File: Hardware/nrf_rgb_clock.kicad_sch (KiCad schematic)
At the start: 23 parts, among them U1 NRF54L15-CAAA-Rx, Y1 32MHz

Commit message: progressed layout
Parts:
- added C10, C11: 4u7 100VDC, Capacitor_SMD:C_1206_3216Metric, symbol Device:C_Small
- added C12: 100n 100VDC, Capacitor_SMD:C_0805_2012Metric, symbol Device:C_Small
- added C13, C14: 22u 6.3V, Capacitor_SMD:C_0805_2012Metric, symbol Device:C_Small
- added C15: 15p, Capacitor_SMD:C_0805_2012Metric, symbol Device:C_Small
- added C16: 22n, Capacitor_SMD:C_0805_2012Metric, symbol Device:C_Small
- added C17, C18: ?p, Capacitor_SMD:C_0201_0603Metric, symbol Device:C_Small
- added D174: ACDBMS2100-HF, Diode_SMD:D_SOD-123F, symbol Device:D_Schottky_Small_Filled
- added J1: Conn_01x02, ProjectFootprints:SHDR4W113P700X508_2X2_1039X1200X1200P, symbol Connector_Generic:Conn_01x02
- added L5: 10u, ProjectFootprints:NRS5040T3R3NMGJV, symbol Device:L_Small
- added R1: 0R, Resistor_SMD:R_0805_2012Metric, symbol Device:R_Small
- added R2: 210k, Resistor_SMD:R_0805_2012Metric, symbol Device:R_Small
- added R3: 68k, Resistor_SMD:R_0805_2012Metric, symbol Device:R_Small
- added R4: 47k, Resistor_SMD:R_0805_2012Metric, symbol Device:R_Small
- added TP1, TP2: TestPoint, TestPoint:TestPoint_THTPad_2.0x2.0mm_Drill1.0mm, symbol Connector:TestPoint
- added U2: MP4562, ProjectFootprints:MP4562, symbol ProjectSymbols:MP4562
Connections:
- net GND: now also C10.2, C11.2, C13.2, C14.2, C16.2, C17.2, C18.2, D174.2 (A), J1.2 (Pin_2), R3.2, R4.2, TP2.1, U2.2 (GND)
- net NRF_RF: now also AE1.1 (FEED), L2.2
- net NRF_XC1: now also Y1.1, C17.1; no longer Y1.3
- net NRF_XC2: now also Y1.3, C18.1; no longer Y1.1
- new net: C12.2, D174.1 (K), L5.1, U2.7 (SW)
- new net: C15.2, R2.2, R3.1, U2.4 (FB)
- new net: R4.1, U2.3 (FREQ)
- new net: C12.1, U2.8 (BST)
- new net: C16.1, U2.1 (SS)
- new net: R1.1, U2.5 (EN)
- new net +3V3: C13.1, C14.1, C15.1, L5.2, R2.1, TP1.1
- new net V_EXT: C10.1, C11.1, J1.1 (Pin_1), R1.2, U2.6 (VIN)
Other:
- note added: "3V3 BUCK"
- note added: "ACDC Converter 48-24Vin"
- note removed: "Power"
- moved on the sheet: AE1, C1, C2, C3, C4, C5, C6, C7, C8, C9, D116, D117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

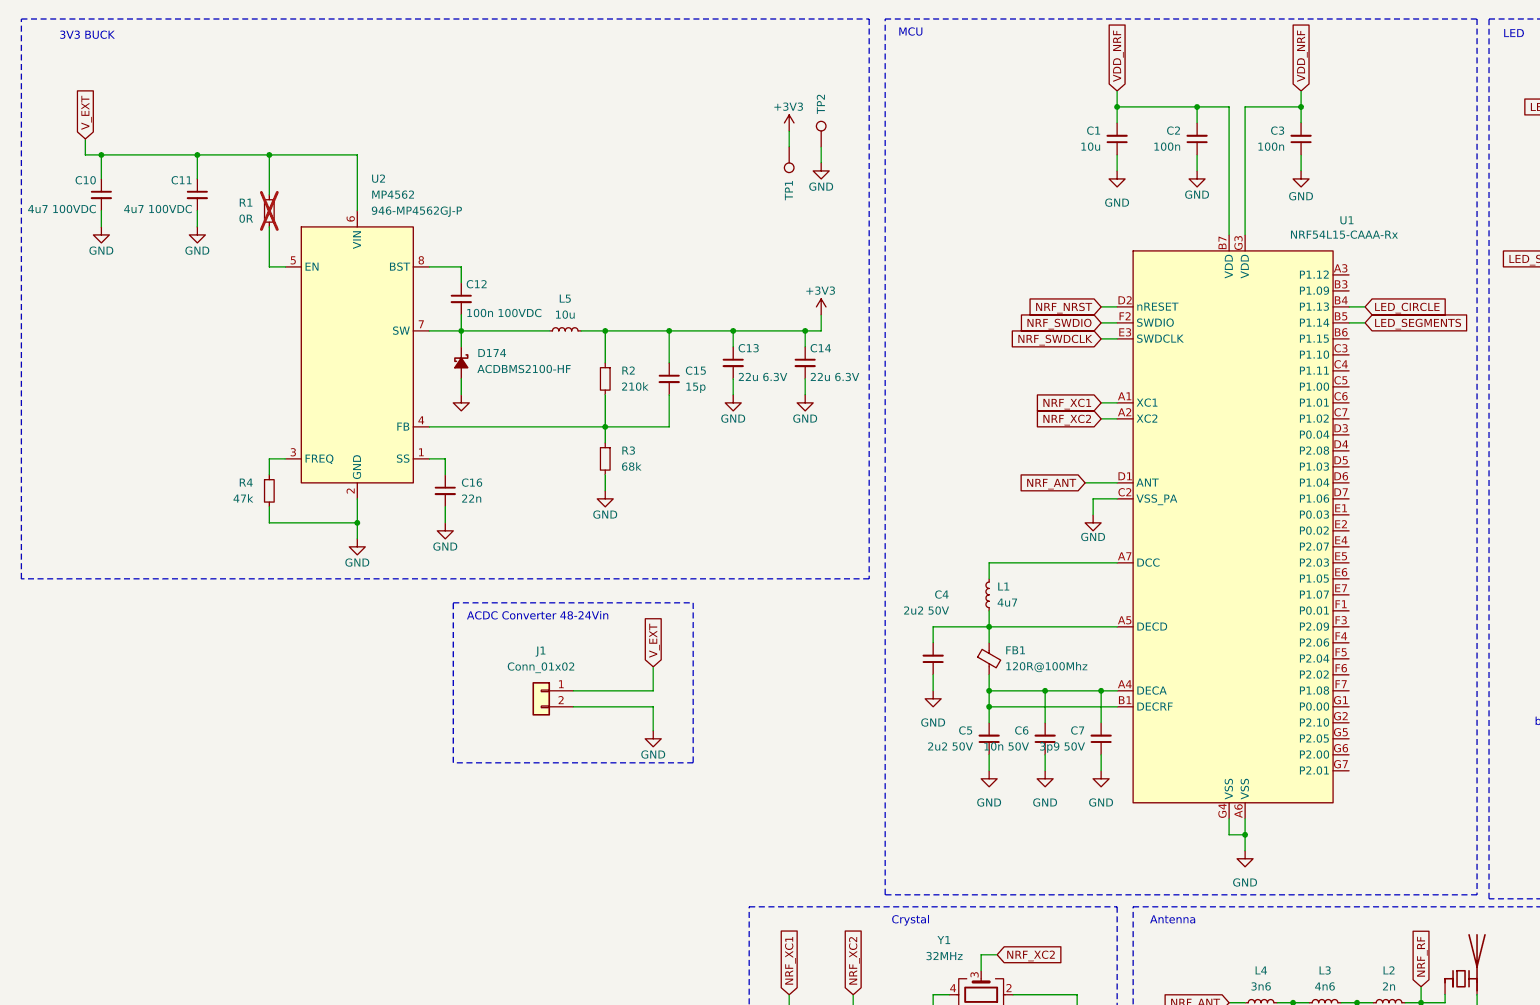
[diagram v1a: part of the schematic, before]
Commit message: layout progress
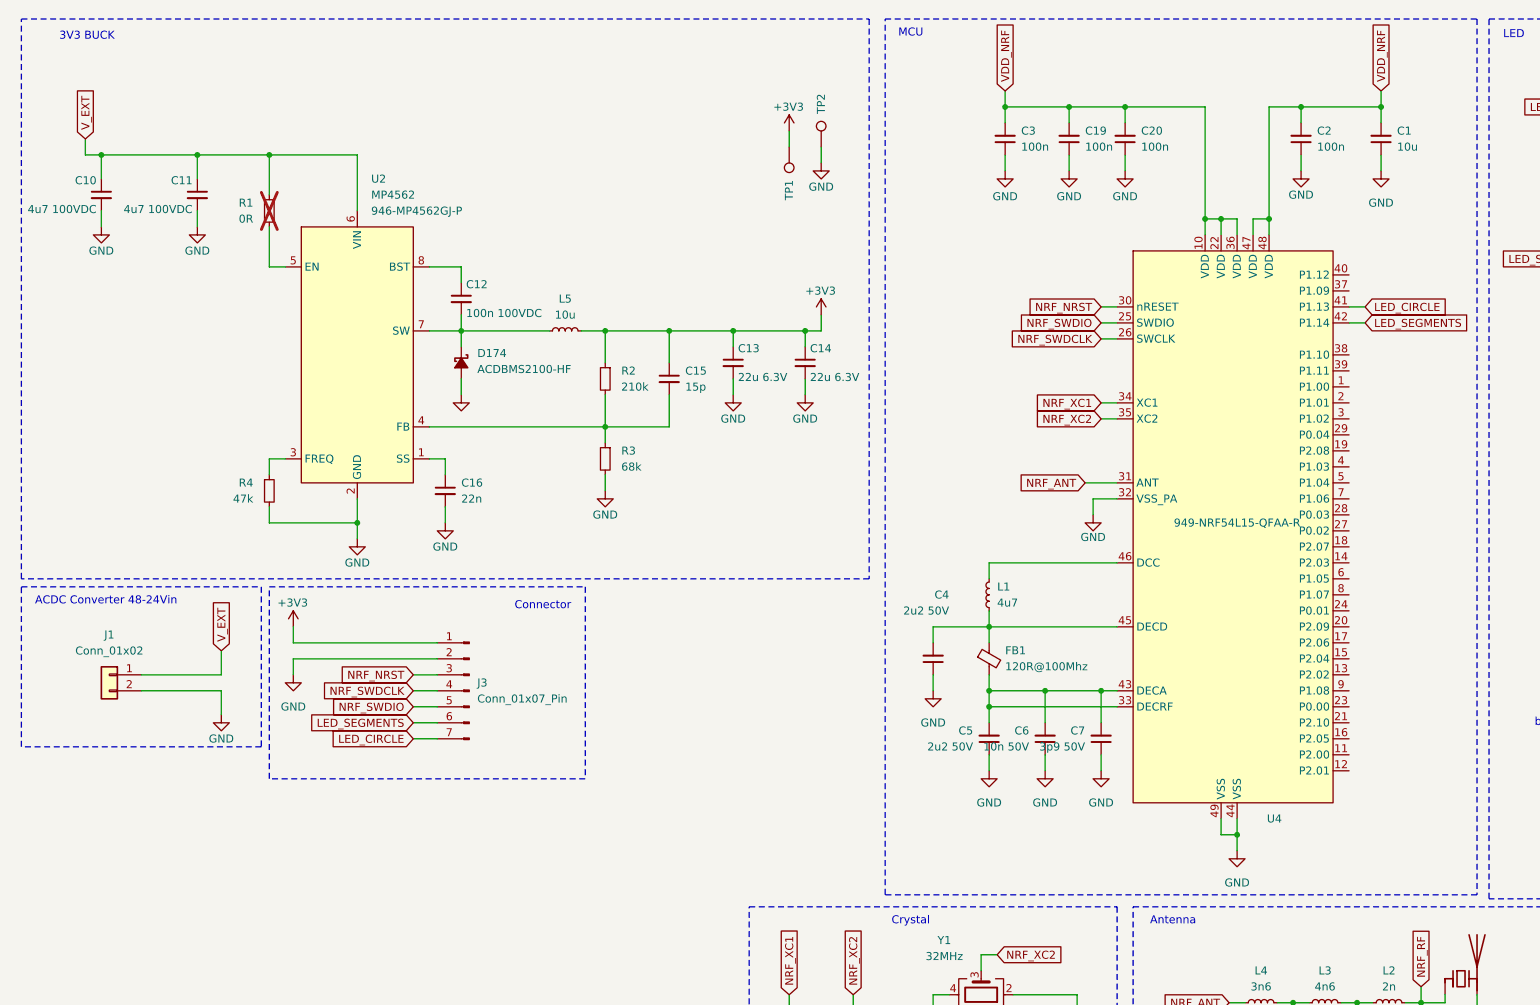
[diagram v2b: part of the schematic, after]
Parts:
- removed U1: NRF54L15-CAAA-Rx, ProjectFootprints:WLCSP 300, symbol ProjectSymbols:nRF54Lxx
- added C19, C20: 100n, Capacitor_SMD:C_0402_1005Metric, symbol Device:C_Small
- added J3: Conn_01x07_Pin, Connector_PinHeader_2.54mm:PinHeader_1x07_P2.54mm_Vertical, symbol Connector:Conn_01x07_Pin
- added U4: ~, ProjectFootprints:QFN-48_EP_6x6_Pitch0.4mm, symbol ProjectSymbols:nRF54L15-QFxx
- L5: LCSC (none) -> C2932476
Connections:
- net +3V3: now also J3.1 (Pin_1)
- net GND: now also C19.1, C20.1, J3.2 (Pin_2), U4.32 (VSS_PA), U4.44 (VSS), U4.49 (VSS)
- net LED_CIRCLE: now also J3.7 (Pin_7), U4.41 (P1.13)
- net LED_SEGMENTS: now also J3.6 (Pin_6), U4.42 (P1.14)
- net NRF_ANT: now also U4.31 (ANT)
- net NRF_NRST: now also J3.3 (Pin_3), U4.30 (nRESET)
- net NRF_SWDCLK: now also J3.4 (Pin_4), U4.26 (SWCLK)
- net NRF_SWDIO: now also J3.5 (Pin_5), U4.25 (SWDIO)
- net NRF_XC1: now also U4.34 (XC1)
- net NRF_XC2: now also U4.35 (XC2)
- net VDD_NRF: now also C19.2, C20.2, U4.10 (VDD), U4.22 (VDD), U4.36 (VDD), U4.47 (VDD), U4.48 (VDD)
- net at C5.2, C6.2, C7.2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: now also U4.33 (DECRF), U4.43 (DECA)
- net at C4.2, FB1.1, L1.2: now also U4.45 (DECD)
- net at L1.1: now also U4.46 (DCC)
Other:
- note added: "Connector"
- moved on the sheet: C1, C2, C3, J1
